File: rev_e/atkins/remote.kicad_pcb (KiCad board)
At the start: 2 copper layers, 91.9 x 69.3 mm, 22 parts, among them J1 Conn_01x18_Female, J11 BME390, J2 Conn_01x18_Female, J3 Conn_01x15_Female, J4 Conn_01x03_Female, J5 Conn_01x04_Female, J9 SCD30, SW1 SW_Push, SW2 SW_Push

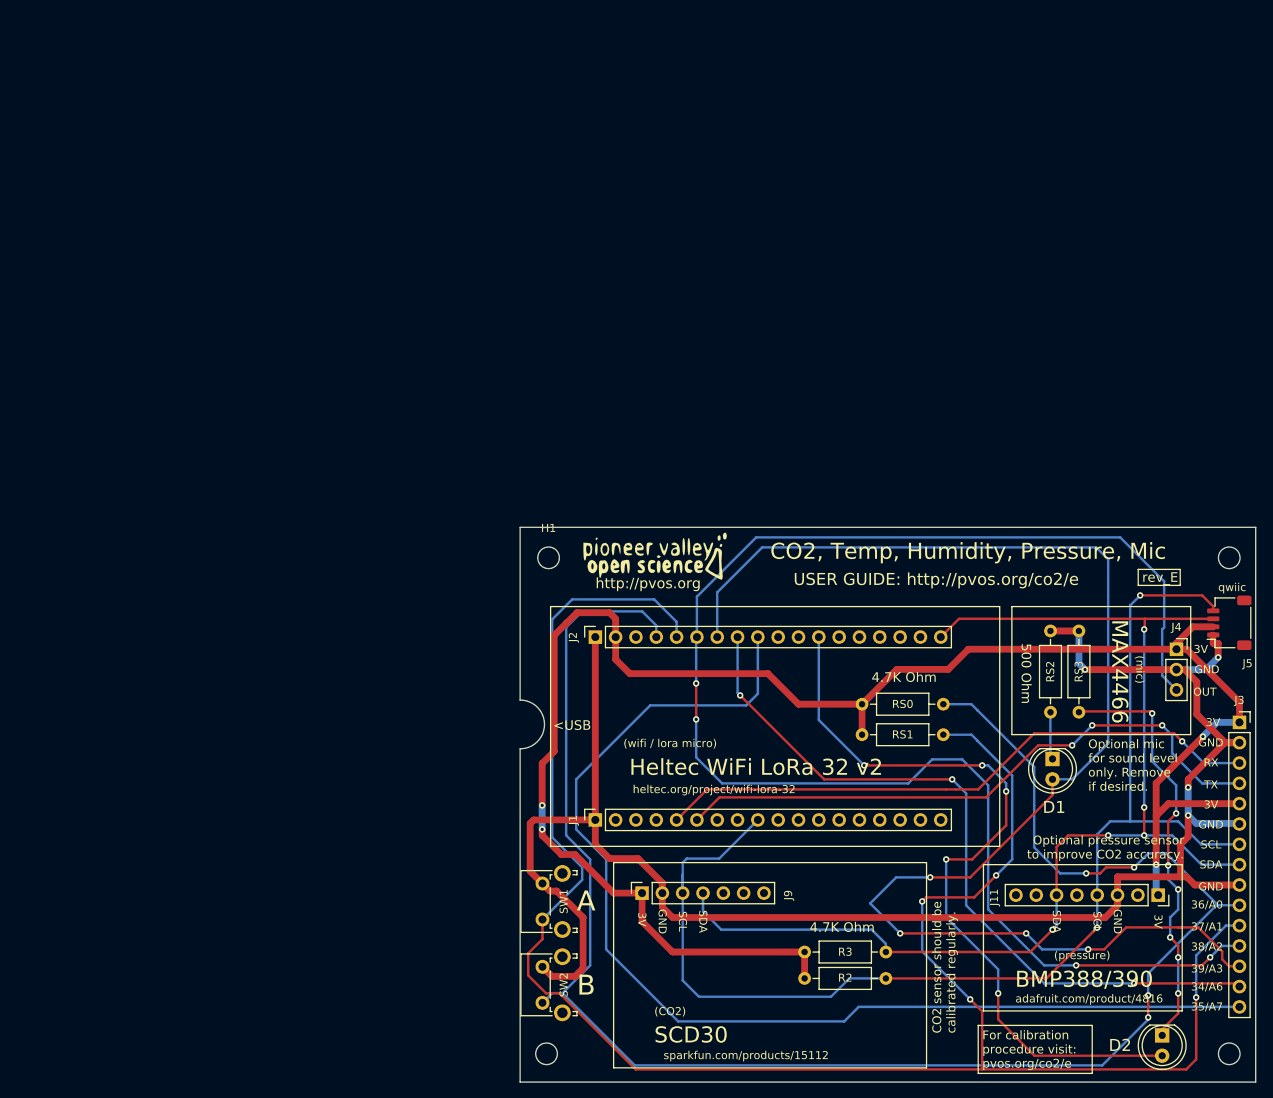
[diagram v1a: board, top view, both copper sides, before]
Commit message: update
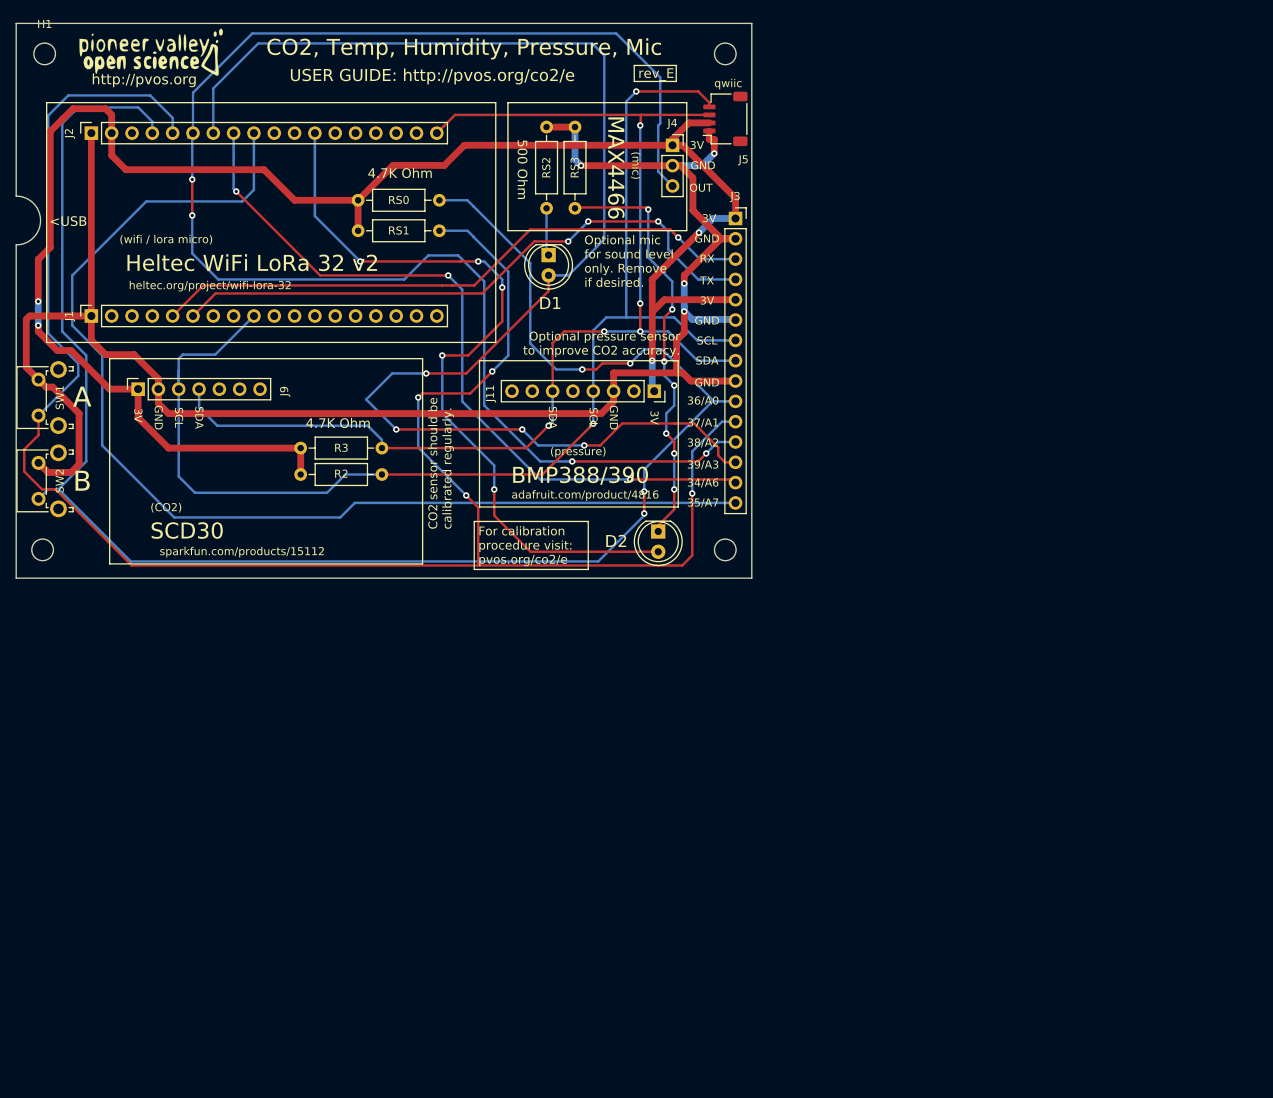
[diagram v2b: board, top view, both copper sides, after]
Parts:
- moved H1 89.1 mm to (3.56, 3.81)
- moved J5 89.1 mm to (88.6, 11.9)
- moved R3 89.1 mm to (35.6, 53.1)
- moved D2 89.1 mm to (80.3, 63.5)
- moved G*** 89.1 mm to (16.8, 3.51)
- moved H2 89.1 mm to (88.6, 3.81)
- moved H3 89.1 mm to (3.30, 65.8)
- moved H4 89.1 mm to (88.6, 65.8)
- moved J1 89.1 mm to (9.40, 36.6)
- moved J2 89.1 mm to (9.40, 13.7)
- moved J3 89.1 mm to (89.9, 24.4)
- moved J9 89.1 mm to (15.2, 45.7)
- moved R2 89.1 mm to (35.6, 56.4)
- moved RS0 89.1 mm to (42.7, 22.1)
- moved RS1 89.1 mm to (42.7, 25.9)
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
